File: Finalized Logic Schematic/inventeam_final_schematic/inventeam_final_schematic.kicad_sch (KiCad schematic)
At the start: 27 parts, among them J1 USB_C_Receptacle_PowerOnly_6P, J2 Conn_01x02, J3 Screw_Terminal_01x04, J4 JST Female, J5 JST Male, J6 JST Female, J7 JST Male, U1 LM66100DCK, U2 LM66100DCK

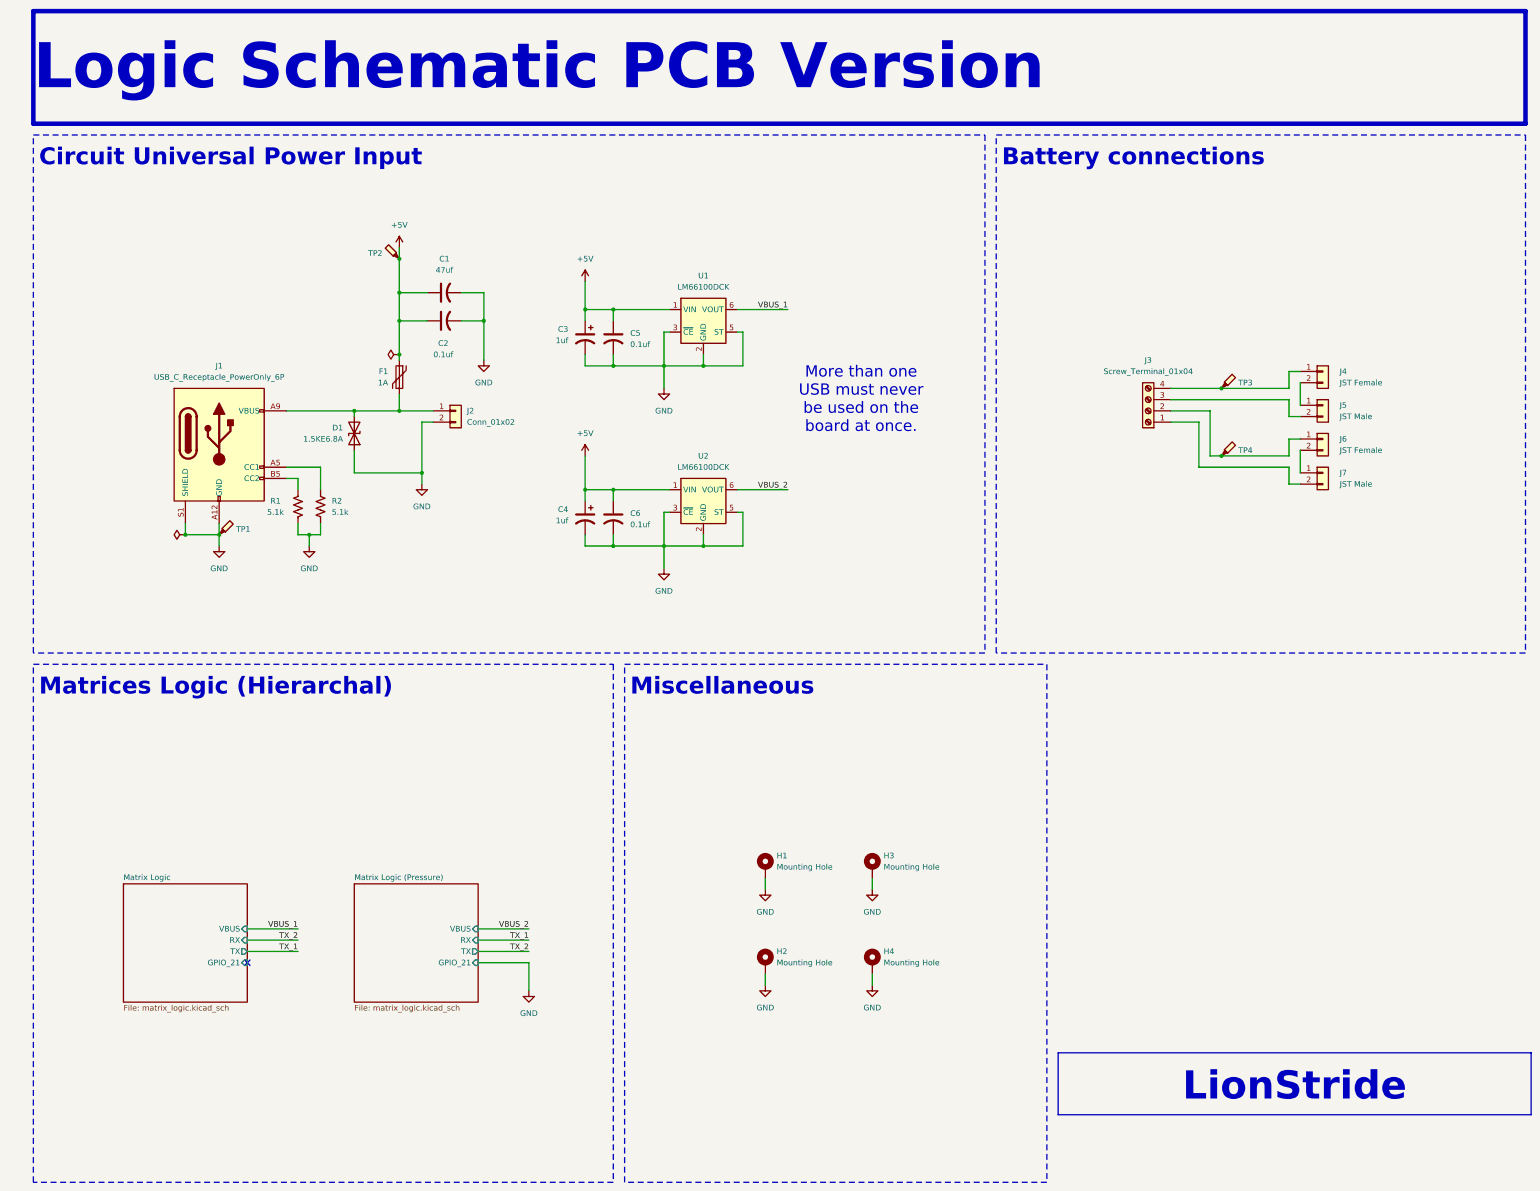
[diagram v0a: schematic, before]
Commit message: Logic schematic V3
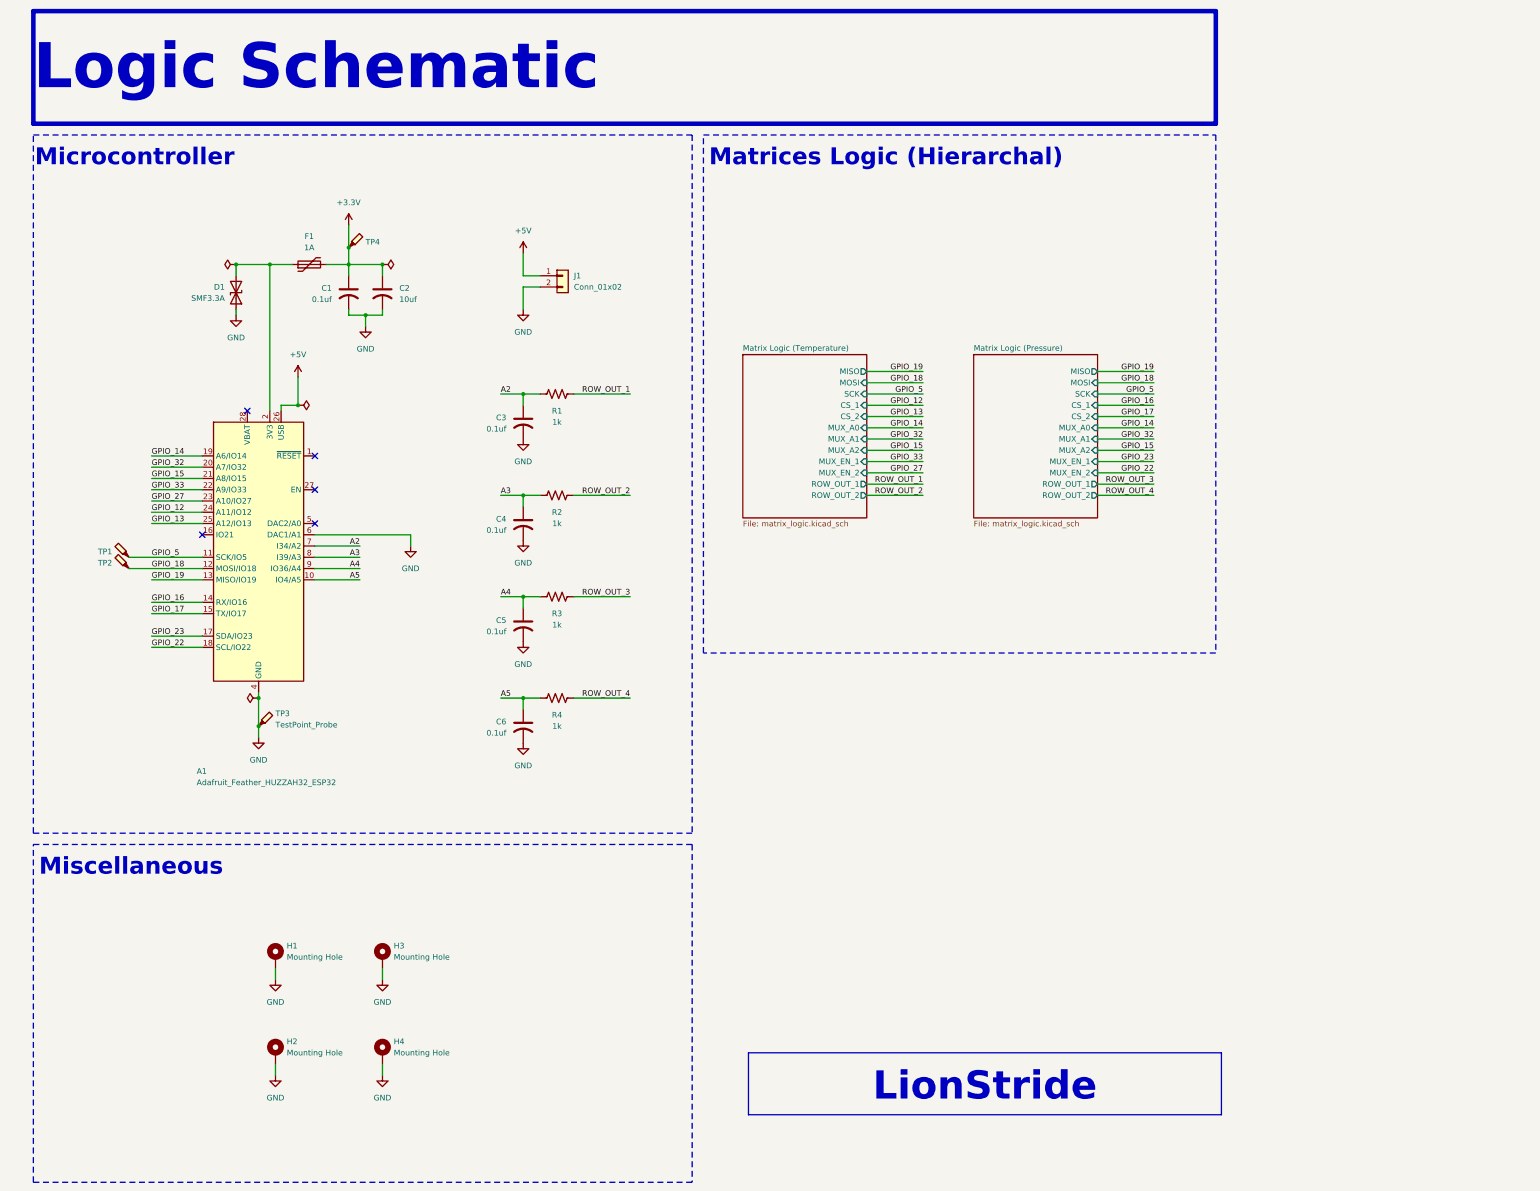
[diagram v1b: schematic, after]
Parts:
- removed C3, C4: 1uf, Capacitor_THT:CP_Axial_L10.0mm_D4.5mm_P15.00mm_Horizontal, symbol Device:C_Polarized_US
- removed J1: USB_C_Receptacle_PowerOnly_6P, Connector_USB:USB_C_Receptacle_GCT_USB4125-xx-x_6P_TopMnt_Horizontal, symbol Connector:USB_C_Receptacle_PowerOnly_6P
- removed J2: Conn_01x02, Connector_PinHeader_2.54mm:PinHeader_1x02_P2.54mm_Vertical, symbol Connector_Generic:Conn_01x02
- removed J3: Screw_Terminal_01x04, TerminalBlock:TerminalBlock_Xinya_XY308-2.54-4P_1x04_P2.54mm_Horizontal, symbol Connector:Screw_Terminal_01x04
- removed J4, J6: JST Female, Connector_PinHeader_2.54mm:PinHeader_1x02_P2.54mm_Vertical, symbol Connector_Generic:Conn_01x02
- removed J5, J7: JST Male, Connector_PinHeader_2.54mm:PinHeader_1x02_P2.54mm_Vertical, symbol Connector_Generic:Conn_01x02
- removed U1, U2: LM66100DCK, Package_TO_SOT_SMD:SOT-363_SC-70-6, symbol Power_Management:LM66100DCK
- added A1: Adafruit_Feather_HUZZAH32_ESP32, Module:Adafruit_Feather, symbol MCU_Module:Adafruit_Feather_HUZZAH32_ESP32
- added C3, C4: 0.1uf, Capacitor_THT:C_Disc_D5.0mm_W2.5mm_P5.00mm, symbol Device:C_US
- added J1: Conn_01x02, Connector_PinHeader_2.54mm:PinHeader_1x02_P2.54mm_Vertical, symbol Connector_Generic:Conn_01x02
- added R3, R4: 1k, Resistor_THT:R_Axial_DIN0207_L6.3mm_D2.5mm_P7.62mm_Horizontal, symbol Device:R_US
- C1: value 47uf -> 0.1uf; footprint Capacitor_THT:CP_Radial_D5.0mm_P2.50mm -> Capacitor_THT:C_Disc_D5.0mm_W2.5mm_P5.00mm
- C2: value 0.1uf -> 10uf; footprint Capacitor_THT:C_Disc_D5.0mm_W2.5mm_P5.00mm -> Capacitor_THT:C_Disc_D5.0mm_W2.5mm_P2.50mm
- D1: value 1.5KE6.8A -> SMF3.3A; footprint Diode_THT:D_DO-201_P15.24mm_Horizontal -> Diode_SMD:D_SOD-123F
- R1, R2: value 5.1k -> 1k
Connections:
- net +5V: now also A1.26 (USB), J1.1 (Pin_1); no longer C1.1, C2.1, C5.1, C6.1, F1.1, TP2.1
- net GND: now also TP3.1, A1.4 (GND), A1.6 (DAC1/A1), C3.2, C4.2, J1.2 (Pin_2); no longer R1.2, R2.2, TP1.1
- net ROW_OUT_1: now reaches R1.1
- net ROW_OUT_2: now reaches R2.1
- net +3.3V: now reaches TP4.1
- net +3.3V: now also C1.1, C2.1, F1.2
- net at D1.2 (A2): now also F1.1, A1.2 (3V3); no longer F1.2
- new net A2: A1.7 (I34/A2), C3.1, R1.2
- new net A3: A1.8 (I39/A3), C4.1, R2.2
- new net A4: A1.9 (IO36/A4), C5.1, R3.2
- new net A5: A1.10 (IO4/A5), C6.1, R4.2
- new net GPIO_12: A1.24 (A11/IO12)
- new net GPIO_13: A1.25 (A12/IO13)
- new net GPIO_14: A1.19 (A6/IO14)
- new net GPIO_15: A1.21 (A8/IO15)
- new net GPIO_16: A1.14 (RX/IO16)
- new net GPIO_17: A1.15 (TX/IO17)
- new net GPIO_18: A1.12 (MOSI/IO18), TP2.1
- new net GPIO_19: A1.13 (MISO/IO19)
- new net GPIO_22: A1.18 (SCL/IO22)
- new net GPIO_23: A1.17 (SDA/IO23)
- new net GPIO_27: A1.23 (A10/IO27)
- new net GPIO_32: A1.20 (A7/IO32)
- new net GPIO_33: A1.22 (A9/IO33)
- new net GPIO_5: A1.11 (SCK/IO5), TP1.1
- new net ROW_OUT_3: R3.1
- new net ROW_OUT_4: R4.1
- no-connect marks 1 -> 5
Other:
- sheet Matrix Logic renamed Matrix Logic (Temperature)
- sheet Matrix Logic (Pressure) ports: added CS_1, CS_2, MISO, MOSI, MUX_A0, MUX_A1, MUX_A2, MUX_EN_1, MUX_EN_2, ROW_OUT_1, ROW_OUT_2, SCK; removed GPIO_21, RX, TX, VBUS
- sheet Matrix Logic (Temperature) ports: added CS_1, CS_2, MISO, MOSI, MUX_A0, MUX_A1, MUX_A2, MUX_EN_1, MUX_EN_2, ROW_OUT_1, ROW_OUT_2, SCK; removed GPIO_21, RX, TX, VBUS
- note added: "Logic Schematic"
- note added: "Microcontroller"
- note removed: "Battery connections"
- note removed: "Circuit Universal Power Input"
- note removed: "Logic Schematic PCB Version"
- note removed: "More than one USB must never be used on the board at once."
- moved on the sheet: H1, H2, H3, H4
